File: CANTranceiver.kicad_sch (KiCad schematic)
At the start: 9 parts, among them U3 IC TRANSCEIVER 1/1 8SO

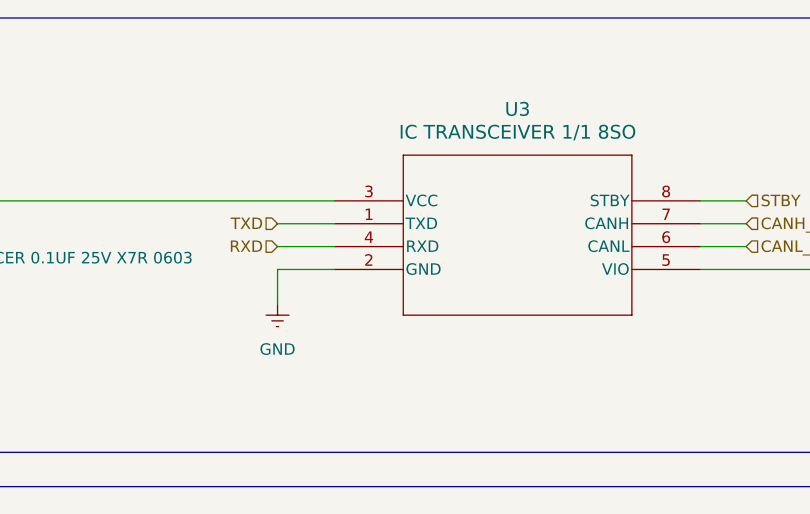
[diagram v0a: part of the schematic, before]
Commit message: minor changes
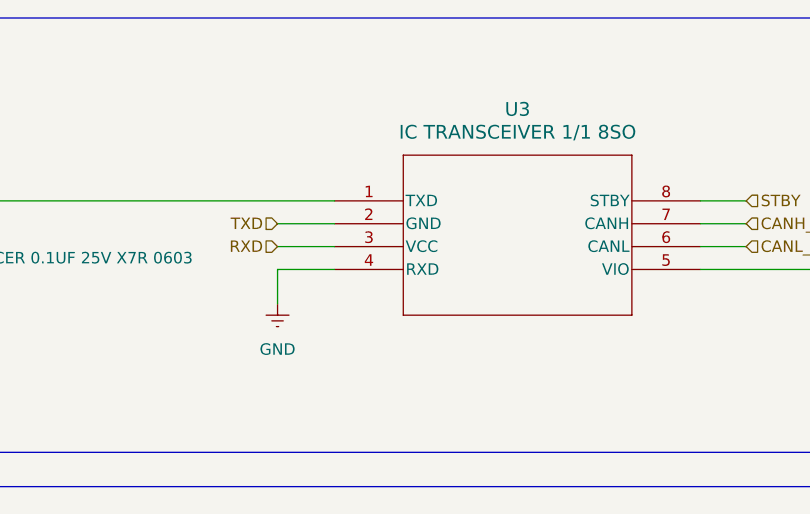
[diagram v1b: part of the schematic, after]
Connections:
- net 5V: now also U3.1 (TXD); no longer U3.3 (VCC)
- net GND: now also U3.4 (RXD); no longer U3.2 (GND)
- net RXD: now also U3.3 (VCC); no longer U3.4 (RXD)
- net TXD: now also U3.2 (GND); no longer U3.1 (TXD)
